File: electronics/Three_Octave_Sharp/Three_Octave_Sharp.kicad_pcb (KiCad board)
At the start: 2 copper layers, 247.7 x 76.2 mm, 110 parts, among them J1 HRO_TYPE-C-31-M-12, SW1 Key Tab, SW10 Key O, SW11 Key P, SW12 Key BS, SW13 Key Caps, SW14 Key A, SW15 Key S, SW16 Key D, SW17 Key F, SW18 Key G, SW19 Key H, SW2 Key Q, SW20 Key J, SW21 Key K, SW22 Key L, SW23 Key Return, SW24 Key Shift, SW25 Key Z, SW26 Key X, SW27 Key C, SW28 Key V, SW29 Key B, SW3 Key W, SW30 Key N, SW31 Key M, SW32 Key ,, SW33 Key Shift, SW34 Key Ctrl, SW35 Key Cmd, SW36 Key Space, SW37 Key Opt, SW38 Key Fn, SW4 Key E, SW5 Key R, SW6 Key T, SW7 Key Y, SW8 Key U, SW9 Key I, U1 Raspberry_Pi_RP2040, U2 W25Q64JVXGIQ, U3 AP2112K-3.3, Y1 12MHz

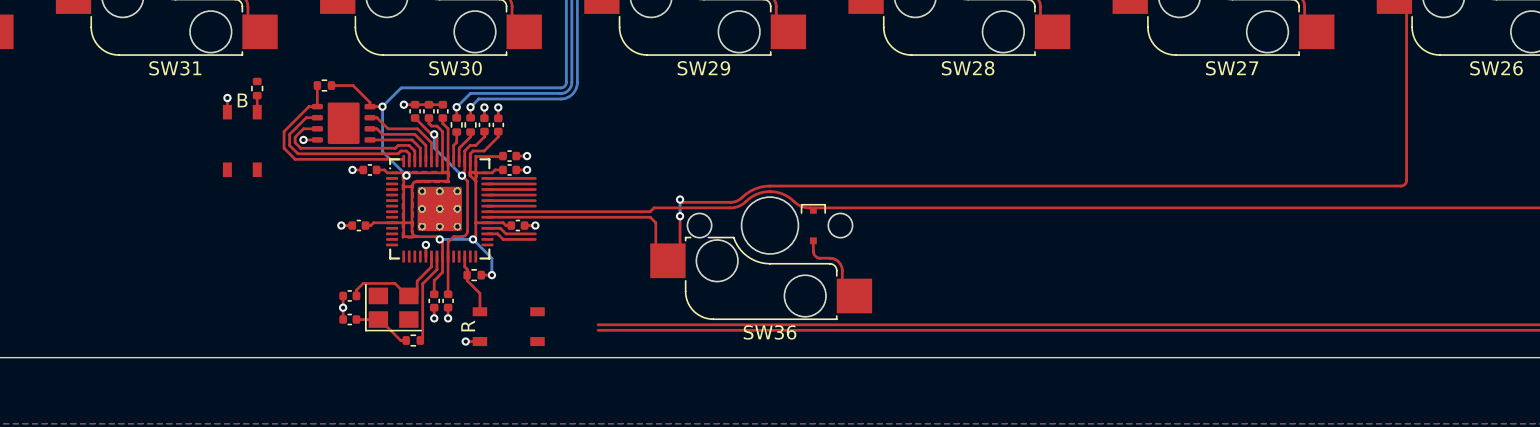
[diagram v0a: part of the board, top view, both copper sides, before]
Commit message: WIP: Update schematic and PCB design
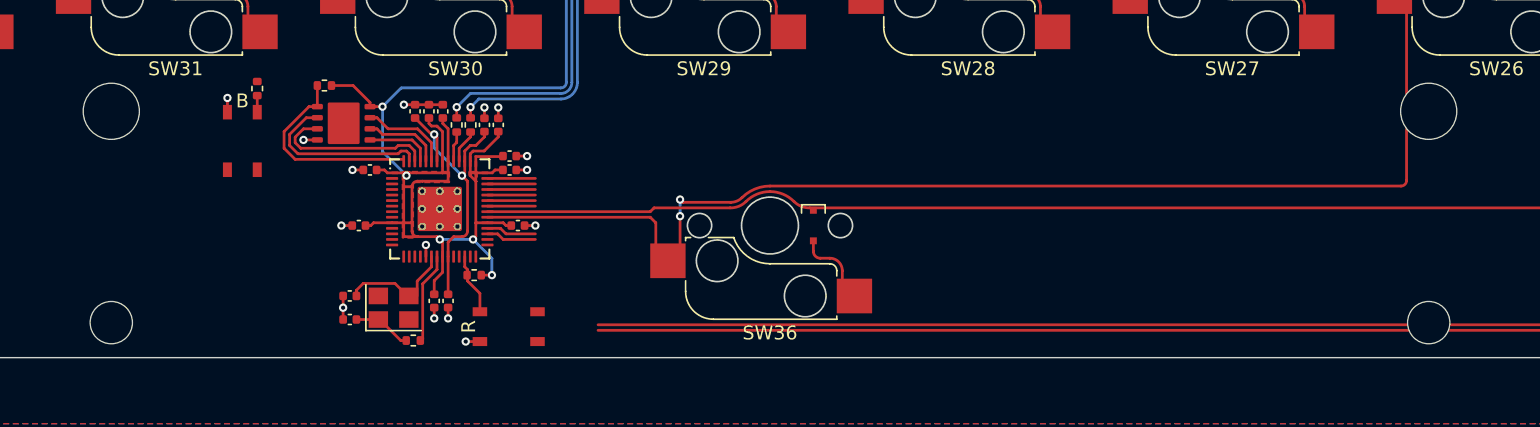
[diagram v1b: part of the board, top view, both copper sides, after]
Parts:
- added REF**: Stabilizer_6u, Project_Library:Stabilizer_6u, F.Cu at (152.4, 95.2)
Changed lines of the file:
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@@
     )
+  )
+  (footprint "Project_Library:Stabilizer_6u" (layer "F.Cu")
+    (at 152.4 95.25 180)
+    (fp_text reference "REF**" (at 0 -0.5 180 unlocked) (layer "F.SilkS") hide
+        (effects (font (size 1 1) (thickness 0.1)))
+    )
+    (fp_text value "Stabilizer_6u" (at 0 1 180 unlocked) (layer "F.Fab") hide
+        (effects (font (size 1 1) (thickness 0.15)))
+    )
+    (fp_text user "${REFERENCE}" (at 0 2.5 180 unlocked) (layer "F.Fab") hide
+        (effects (font (size 1 1) (thickness 0.15)))
+    )
+    (fp_rect (start -57.15 -9.525) (end 57.15 9.525)
+      (stroke (width 0.12) (type solid)) (fill none) (layer "F.Fab"))
+    (fp_rect (start -51 -9) (end -44 9)
+      (stroke (width 0.1) (type default)) (fill none) (layer "F.Fab"))
+    (fp_rect (start -7.8 -7.8) (end 7.8 7.8)
+      (stroke (width 0.12) (type solid)) (fill none) (layer "F.Fab"))
+    (fp_rect (start 44 -9) (end 51 9)
+      (stroke (width 0.1) (type default)) (fill none) (layer "F.Fab"))
+    (pad "" np_thru_hole circle (at -47.5 -7 180) (size 3.05 3.05) (drill 3.05) (layers "F&B.Cu" "*.Mask"))
+    (pad "" np_thru_hole circle (at -47.5 8.24 180) (size 4.05 4.05) (drill 4.05) (layers "F&B.Cu" "*.Mask"))
+    (pad "" np_thru_hole circle (at 47.5 -7 180) (size 3.05 3.05) (drill 3.05) (layers "F&B.Cu" "*.Mask"))
+    (pad "" np_thru_hole circle (at 47.5 8.24 180) (size 4.05 4.05) (drill 4.05) (layers "F&B.Cu" "*.Mask"))
   )
   (footprint "Capacitor_SMD:C_0402_1005Metric" (layer "F.Cu")

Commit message: WIP: Update PCB design
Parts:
- removed the REF** at (50.0, 57.1)
- removed the REF** at (254.8, 76.2)
- moved D1 20.5 mm to (250.8, 38.1), turned to -90 degrees
- moved D2 16.0 mm to (231.7, 38.1), turned to -90 degrees
- moved D4 16.0 mm to (193.6, 38.1), turned to -90 degrees
- moved D5 16.0 mm to (174.6, 38.1), turned to -90 degrees
- moved D9 16.0 mm to (98.4, 38.1), turned to -90 degrees
- moved D10 16.0 mm to (79.3, 38.1), turned to -90 degrees
- moved D11 16.0 mm to (60.3, 38.1), turned to -90 degrees
- moved D8 16.0 mm to (117.4, 38.1), turned to -90 degrees
- moved D3 16.0 mm to (212.7, 38.1), turned to -90 degrees
- moved D34 14.3 mm to (234.1, 95.2)
- moved D35 14.3 mm to (210.3, 95.2)
- moved SW1 14.3 mm to (247.0, 41.9)
- moved D24 14.3 mm to (243.6, 76.2)
- moved D36 14.3 mm to (141.2, 95.2)
- moved REF** 14.3 mm to (138.1, 95.2)
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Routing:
- net COL3: track 51.7 -> 112.5 mm, vias 6 -> 4
- net COL8: track 0.00 -> 49.7 mm, vias 0 -> 4
- net COL7: track 0.00 -> 49.7 mm, vias 0 -> 4
- net COL6: track 0.00 -> 49.7 mm, vias 0 -> 6
- net COL4: track 51.7 -> 93.0 mm, vias 6 -> 4
- net COL9: track 0.00 -> 21.9 mm, vias 0 -> 2
- net COL5: track 66.7 -> 51.7 mm
- net ROW0: track 222.5 -> 211.6 mm
- net ROW3: track 141.9 -> 132.4 mm
- net ROW1: track 224.7 -> 215.2 mm
- net COL1: track 156.0 -> 164.3 mm, vias 8 -> 6
- net ROW2: track 208.3 -> 203.5 mm
- net COL0: track 180.2 -> 184.6 mm, vias 8 -> 6
- net Net-(D2-A): track 2.28 -> 5.41 mm
- net Net-(D10-A): track 2.28 -> 5.41 mm
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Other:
- board size 247.7 x 76.2 mm -> 228.6 x 76.2 mm
